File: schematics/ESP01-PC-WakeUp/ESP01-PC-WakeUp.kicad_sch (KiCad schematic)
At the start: 18 parts, among them J1 JUSB, J2 JUSB, J3 Pin selector, J4 Power, J5 Out 1, J6 Out 2, Q1 BC337, Q2 2N7000, U1 ESP-01, U2 PS2561

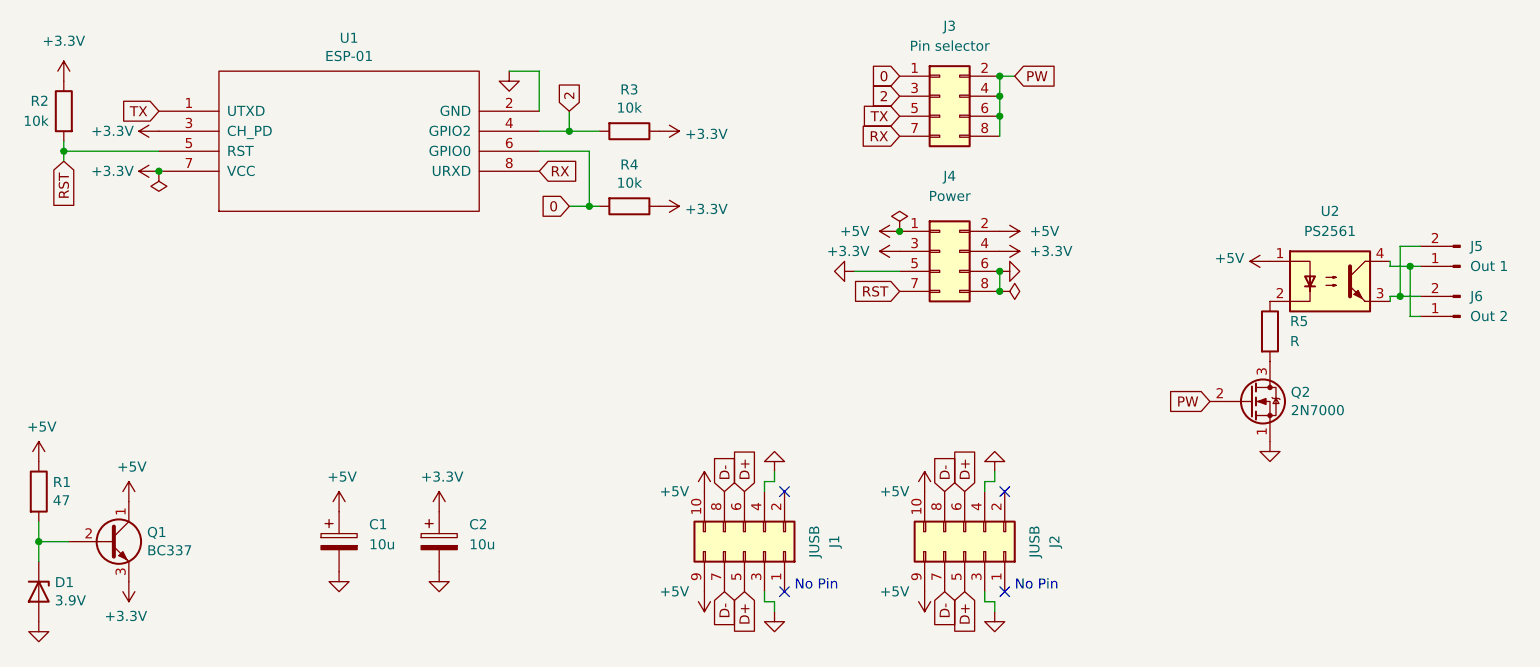
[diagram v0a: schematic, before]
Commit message: feat: first PCB release.
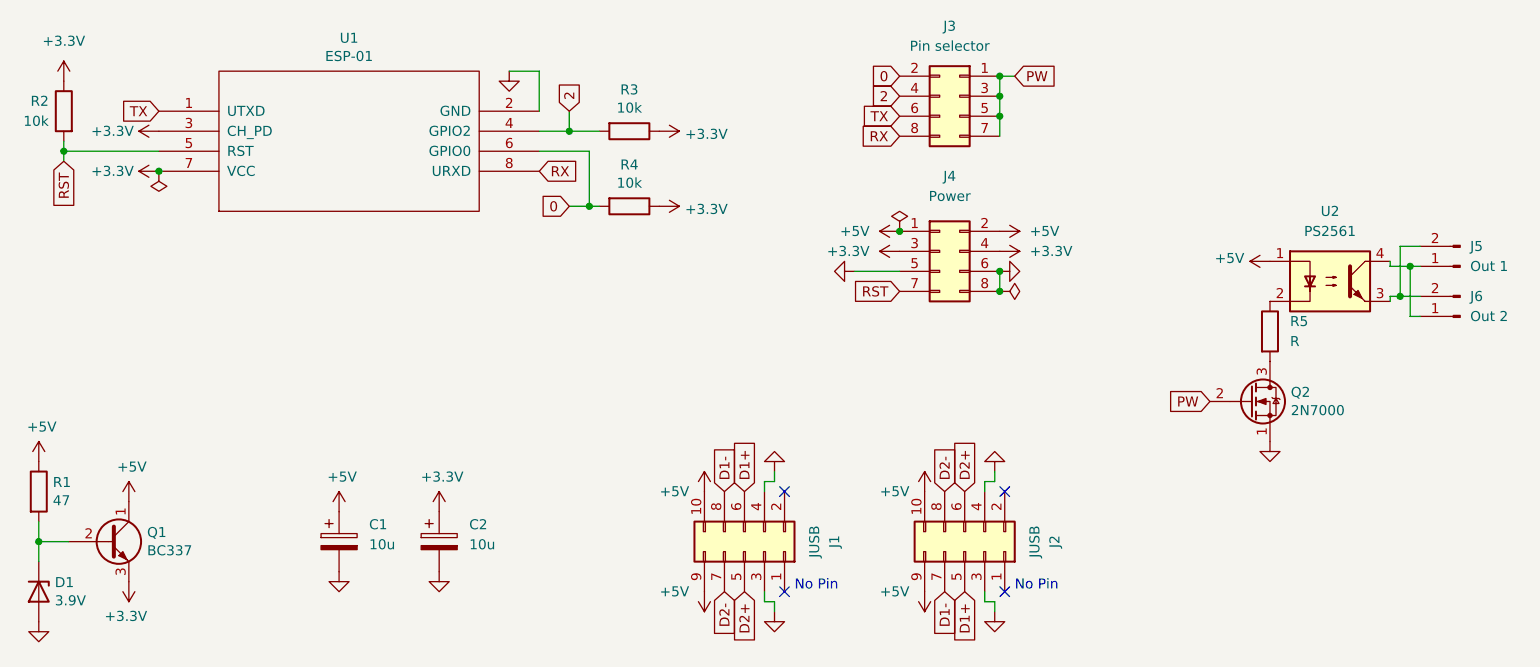
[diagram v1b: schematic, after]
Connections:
- net 0: now also J3.2 (Pin_2); no longer J3.1 (Pin_1)
- net 2: now also J3.4 (Pin_4); no longer J3.3 (Pin_3)
- net PW: now also J3.1 (Pin_1), J3.3 (Pin_3), J3.5 (Pin_5), J3.7 (Pin_7); no longer J3.2 (Pin_2), J3.4 (Pin_4), J3.6 (Pin_6), J3.8 (Pin_8)
- net RX: now also J3.8 (Pin_8); no longer J3.7 (Pin_7)
- net TX: now also J3.6 (Pin_6); no longer J3.5 (Pin_5)
- net D+ renamed D1+
- net D1+: no longer J1.5 (Pin_5), J2.6 (Pin_6)
- net D- renamed D1-
- net D1-: no longer J1.7 (Pin_7), J2.8 (Pin_8)
- new net D2+: J1.5 (Pin_5), J2.6 (Pin_6)
- new net D2-: J1.7 (Pin_7), J2.8 (Pin_8)
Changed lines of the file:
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@@
     )
   )
-  (global_label "D+" (shape input) (at 130.175 102.87 270) (fields_autoplaced)
-    (effects (font (size 1.27 1.27)) (justify right))
-    (property "Intersheet References" "${INTERSHEET_REFS}" (id 0) (at 130.2544 108.1255 90)
+  (global_label "D2+" (shape input) (at 130.175 102.87 270) (fields_autoplaced)
+    (effects (font (size 1.27 1.27)) (justify right))
+    (property "Intersheet References" "${INTERSHEET_REFS}" (id 0) (at 130.0956 109.335 90)
       (effects (font (size 1.27 1.27)) (justify right) hide)
     )
@@
     )
   )
-  (global_label "D-" (shape input) (at 155.575 102.87 270) (fields_autoplaced)
-    (effects (font (size 1.27 1.27)) (justify right))
-    (property "Intersheet References" "${INTERSHEET_REFS}" (id 0) (at 155.6544 108.1255 90)
+  (global_label "D1-" (shape input) (at 155.575 102.87 270) (fields_autoplaced)
+    (effects (font (size 1.27 1.27)) (justify right))
+    (property "Intersheet References" "${INTERSHEET_REFS}" (id 0) (at 155.4956 109.335 90)
       (effects (font (size 1.27 1.27)) (justify right) hide)
     )
@@
     )
   )
-  (global_label "D+" (shape input) (at 130.175 90.17 90) (fields_autoplaced)
+  (global_label "D1+" (shape input) (at 130.175 90.17 90) (fields_autoplaced)
     (effects (font (size 1.27 1.27)) (justify left))
-    (property "Intersheet References" "${INTERSHEET_REFS}" (id 0) (at 130.0956 84.9145 90)
+    (property "Intersheet References" "${INTERSHEET_REFS}" (id 0) (at 130.0956 83.705 90)
       (effects (font (size 1.27 1.27)) (justify left) hide)
     )
   )
-  (global_label "D-" (shape input) (at 127.635 102.87 270) (fields_autoplaced)
-    (effects (font (size 1.27 1.27)) (justify right))
-    (property "Intersheet References" "${INTERSHEET_REFS}" (id 0) (at 127.7144 108.1255 90)
+  (global_label "D2-" (shape input) (at 127.635 102.87 270) (fields_autoplaced)
+    (effects (font (size 1.27 1.27)) (justify right))
+    (property "Intersheet References" "${INTERSHEET_REFS}" (id 0) (at 127.5556 109.335 90)
       (effects (font (size 1.27 1.27)) (justify right) hide)
     )
@@
     )
   )
-  (global_label "D+" (shape input) (at 158.115 90.17 90) (fields_autoplaced)
+  (global_label "D2+" (shape input) (at 158.115 90.17 90) (fields_autoplaced)
     (effects (font (size 1.27 1.27)) (justify left))
-    (property "Intersheet References" "${INTERSHEET_REFS}" (id 0) (at 158.0356 84.9145 90)
+    (property "Intersheet References" "${INTERSHEET_REFS}" (id 0) (at 158.0356 83.705 90)
       (effects (font (size 1.27 1.27)) (justify left) hide)
     )
   )
-  (global_label "D-" (shape input) (at 127.635 90.17 90) (fields_autoplaced)
+  (global_label "D1-" (shape input) (at 127.635 90.17 90) (fields_autoplaced)
     (effects (font (size 1.27 1.27)) (justify left))
-    (property "Intersheet References" "${INTERSHEET_REFS}" (id 0) (at 127.5556 84.9145 90)
+    (property "Intersheet References" "${INTERSHEET_REFS}" (id 0) (at 127.5556 83.705 90)
       (effects (font (size 1.27 1.27)) (justify left) hide)
     )
@@
     )
   )
-  (global_label "D-" (shape input) (at 155.575 90.17 90) (fields_autoplaced)
+  (global_label "D2-" (shape input) (at 155.575 90.17 90) (fields_autoplaced)
     (effects (font (size 1.27 1.27)) (justify left))
-    (property "Intersheet References" "${INTERSHEET_REFS}" (id 0) (at 155.4956 84.9145 90)
+    (property "Intersheet References" "${INTERSHEET_REFS}" (id 0) (at 155.4956 83.705 90)
       (effects (font (size 1.27 1.27)) (justify left) hide)
     )
   )
-  (global_label "D+" (shape input) (at 158.115 102.87 270) (fields_autoplaced)
-    (effects (font (size 1.27 1.27)) (justify right))
-    (property "Intersheet References" "${INTERSHEET_REFS}" (id 0) (at 158.1944 108.1255 90)
+  (global_label "D1+" (shape input) (at 158.115 102.87 270) (fields_autoplaced)
+    (effects (font (size 1.27 1.27)) (justify right))
+    (property "Intersheet References" "${INTERSHEET_REFS}" (id 0) (at 158.0356 109.335 90)
       (effects (font (size 1.27 1.27)) (justify right) hide)
     )
@@
     (pin "8")
   )
-  (symbol (lib_id "Connector_Generic:Conn_02x04_Odd_Even") (at 154.94 40.005 0) (unit 1)
+  (symbol (lib_id "Connector_Generic:Conn_02x04_Odd_Even") (at 157.48 40.005 0) (mirror y) (unit 1)
     (in_bom yes) (on_board yes) (fields_autoplaced)
     (property "Reference" "J3" (id 0) (at 156.21 31.115 0))
     (property "Value" "Pin selector" (id 1) (at 156.21 33.655 0))
-    (property "Footprint" "Connector_PinHeader_2.54mm:PinHeader_2x04_P2.54mm_Vertical" (id 2) (at 154.94 40.005 0)
-      (effects (font (size 1.27 1.27)) hide)
-    )
-    (property "Datasheet" "~" (id 3) (at 154.94 40.005 0)
-      (effects (font (size 1.27 1.27)) hide)
-    )
+    (property "Footprint" "Connector_PinHeader_2.54mm:PinHeader_2x04_P2.54mm_Vertical" (id 2) (at 157.48 40.005 0)
+      (effects (font (size 1.27 1.27)) hide)
+    )
+    (property "Datasheet" "~" (id 3) (at 157.48 40.005 0)
+      (effects (font (size 1.27 1.27)) hide)
+    )
